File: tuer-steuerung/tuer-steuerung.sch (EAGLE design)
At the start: 47 parts, among them IC1 L6203, IC2 MEGA8-P, Q1 16Mhz, T1 BC337, T2 BC337

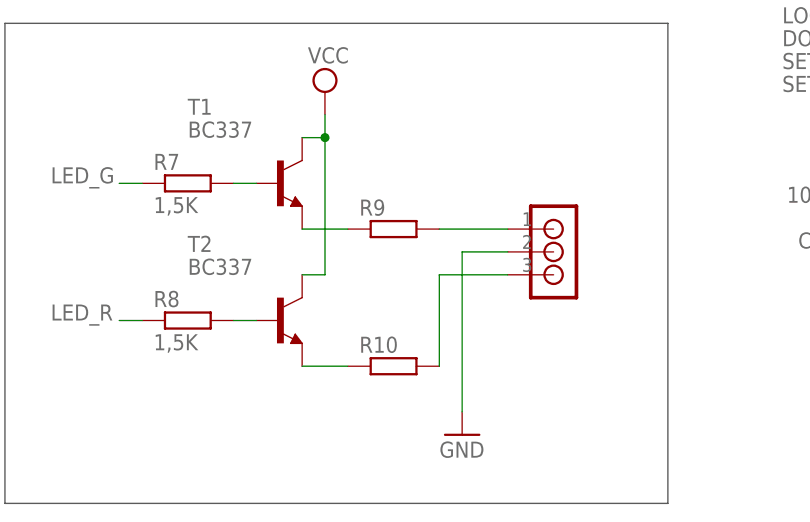
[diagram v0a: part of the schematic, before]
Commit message: Letzte Anpassungen vor dem Ätzen
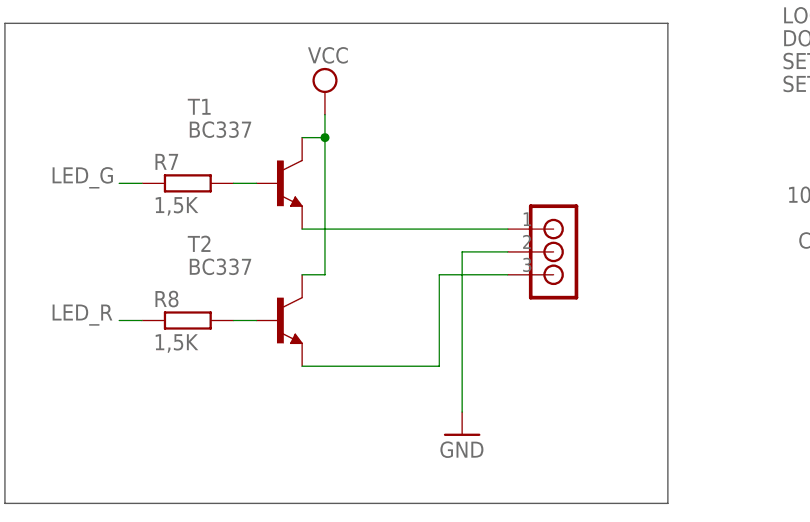
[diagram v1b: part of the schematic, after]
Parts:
- removed R10, R9: (no value), resistor:R-EU_0207/2V
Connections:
- removed net N$12: R9.2, U$4.1
- removed net N$14: R10.2, U$4.3
- net N$11: now also U$4.1; no longer R9.1
- net N$13: now also U$4.3; no longer R10.1
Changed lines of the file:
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@@
 <part name="R8" library="resistor" deviceset="R-EU_" device="0204/5" value="1,5K"/>
 <part name="GND10" library="supply1" deviceset="GND" device=""/>
-<part name="R9" library="resistor" deviceset="R-EU_" device="0207/2V"/>
-<part name="R10" library="resistor" deviceset="R-EU_" device="0207/2V"/>
 <part name="C6" library="resistor" deviceset="C-EU" device="050-025X075" value="12p"/>
 <part name="C7" library="resistor" deviceset="C-EU" device="050-025X075" value="12p"/>
@@
 <instance part="R8" gate="G$1" x="7.62" y="-81.28"/>
 <instance part="GND10" gate="1" x="38.1" y="-93.98"/>
-<instance part="R9" gate="G$1" x="30.48" y="-71.12"/>
-<instance part="R10" gate="G$1" x="30.48" y="-86.36"/>
 <instance part="C6" gate="G$1" x="195.58" y="15.24" rot="R90"/>
 <instance part="C7" gate="G$1" x="195.58" y="5.08" rot="R90"/>
@@
 <segment>
 <pinref part="T1" gate="G$1" pin="E"/>
-<pinref part="R9" gate="G$1" pin="1"/>
-<wire x1="20.32" y1="-71.12" x2="25.4" y2="-71.12" width="0.1524" layer="91"/>
-</segment>
-</net>
-<net name="N$12" class="0">
-<segment>
-<pinref part="R9" gate="G$1" pin="2"/>
-<wire x1="35.56" y1="-71.12" x2="43.18" y2="-71.12" width="0.1524" layer="91"/>
 <pinref part="U$4" gate="G$1" pin="1"/>
+<wire x1="20.32" y1="-71.12" x2="43.18" y2="-71.12" width="0.1524" layer="91"/>
 </segment>
 </net>
@@
 <segment>
 <pinref part="T2" gate="G$1" pin="E"/>
-<pinref part="R10" gate="G$1" pin="1"/>
-<wire x1="20.32" y1="-86.36" x2="25.4" y2="-86.36" width="0.1524" layer="91"/>
-</segment>
-</net>
-<net name="N$14" class="0">
-<segment>
-<pinref part="R10" gate="G$1" pin="2"/>
 <wire x1="35.56" y1="-86.36" x2="35.56" y2="-76.2" width="0.1524" layer="91"/>
 <wire x1="35.56" y1="-76.2" x2="43.18" y2="-76.2" width="0.1524" layer="91"/>
 <pinref part="U$4" gate="G$1" pin="3"/>
-</segment>
-</net>
+<wire x1="20.32" y1="-86.36" x2="35.56" y2="-86.36" width="0.1524" layer="91"/>
+</segment>
+</net>
